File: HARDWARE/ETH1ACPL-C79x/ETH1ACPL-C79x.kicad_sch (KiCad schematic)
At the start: 5 parts

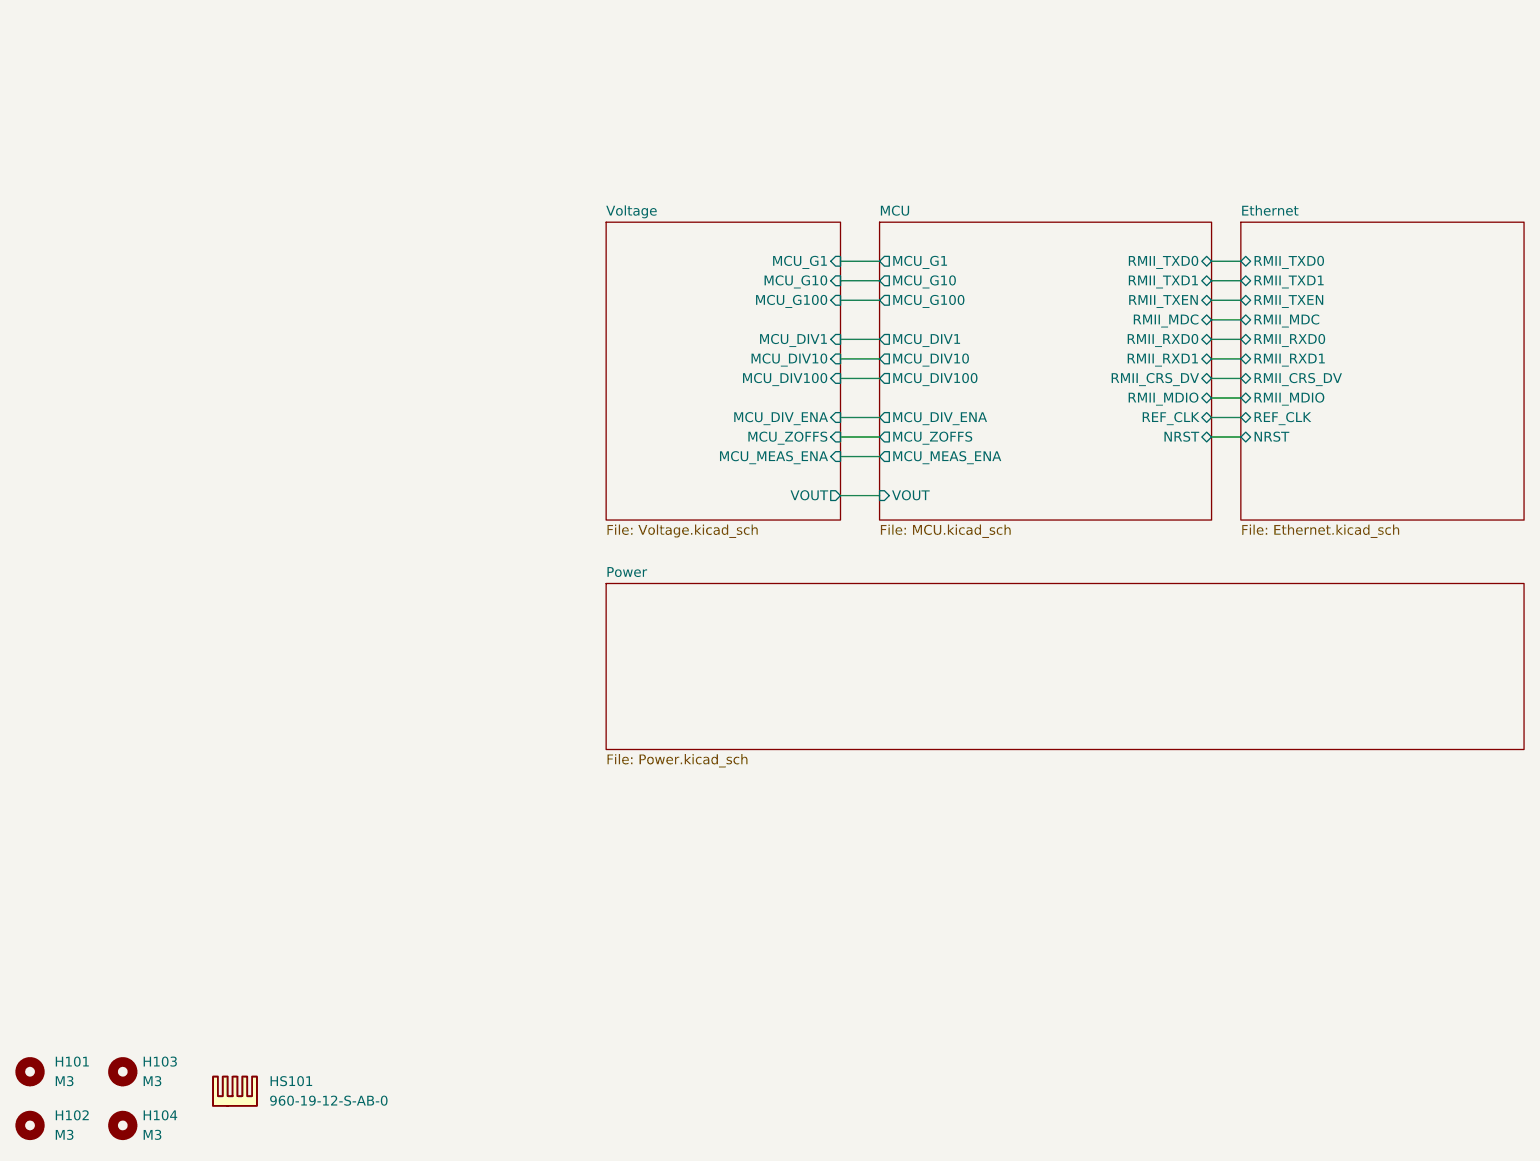
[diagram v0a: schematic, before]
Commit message: Development
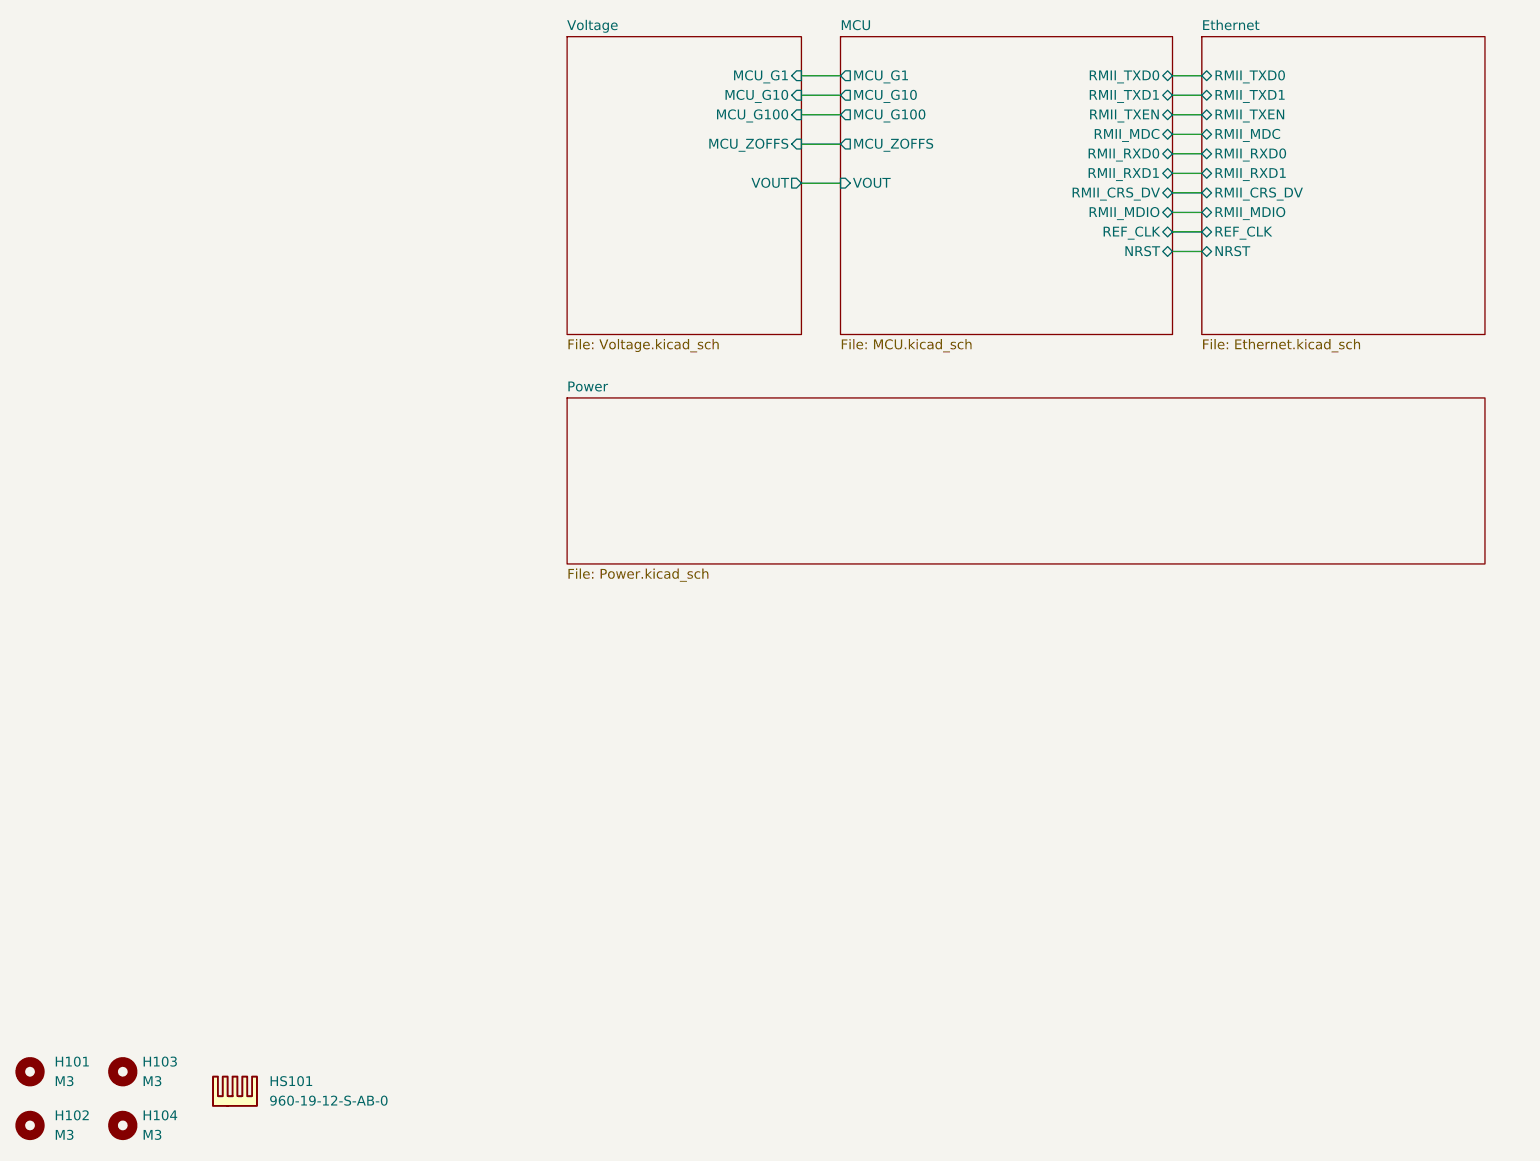
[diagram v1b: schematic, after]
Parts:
- H101, H103: footprint MountingHole:MountingHole_3.2mm_M3_DIN965_Pad -> MountingHole:MountingHole_3.2mm_M3_DIN965
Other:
- sheet MCU ports: added none; removed MCU_DIV1, MCU_DIV10, MCU_DIV100, MCU_DIV_ENA, MCU_MEAS_ENA
- sheet Voltage ports: added none; removed MCU_DIV1, MCU_DIV10, MCU_DIV100, MCU_DIV_ENA, MCU_MEAS_ENA
